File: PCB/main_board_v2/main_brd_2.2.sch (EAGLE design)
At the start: 53 parts, among them J2 SD-card Adapter, J3 E-paper Module, J4 Zigbee Module, J5 BATT, J6 CHARGER, J7 POGO_PINS, J8 ST-LINK, J9 additional I2C bus, U1 STM32F103C8T6-MODULE, U2 LF411CP, U3 TS5A4595DCKR

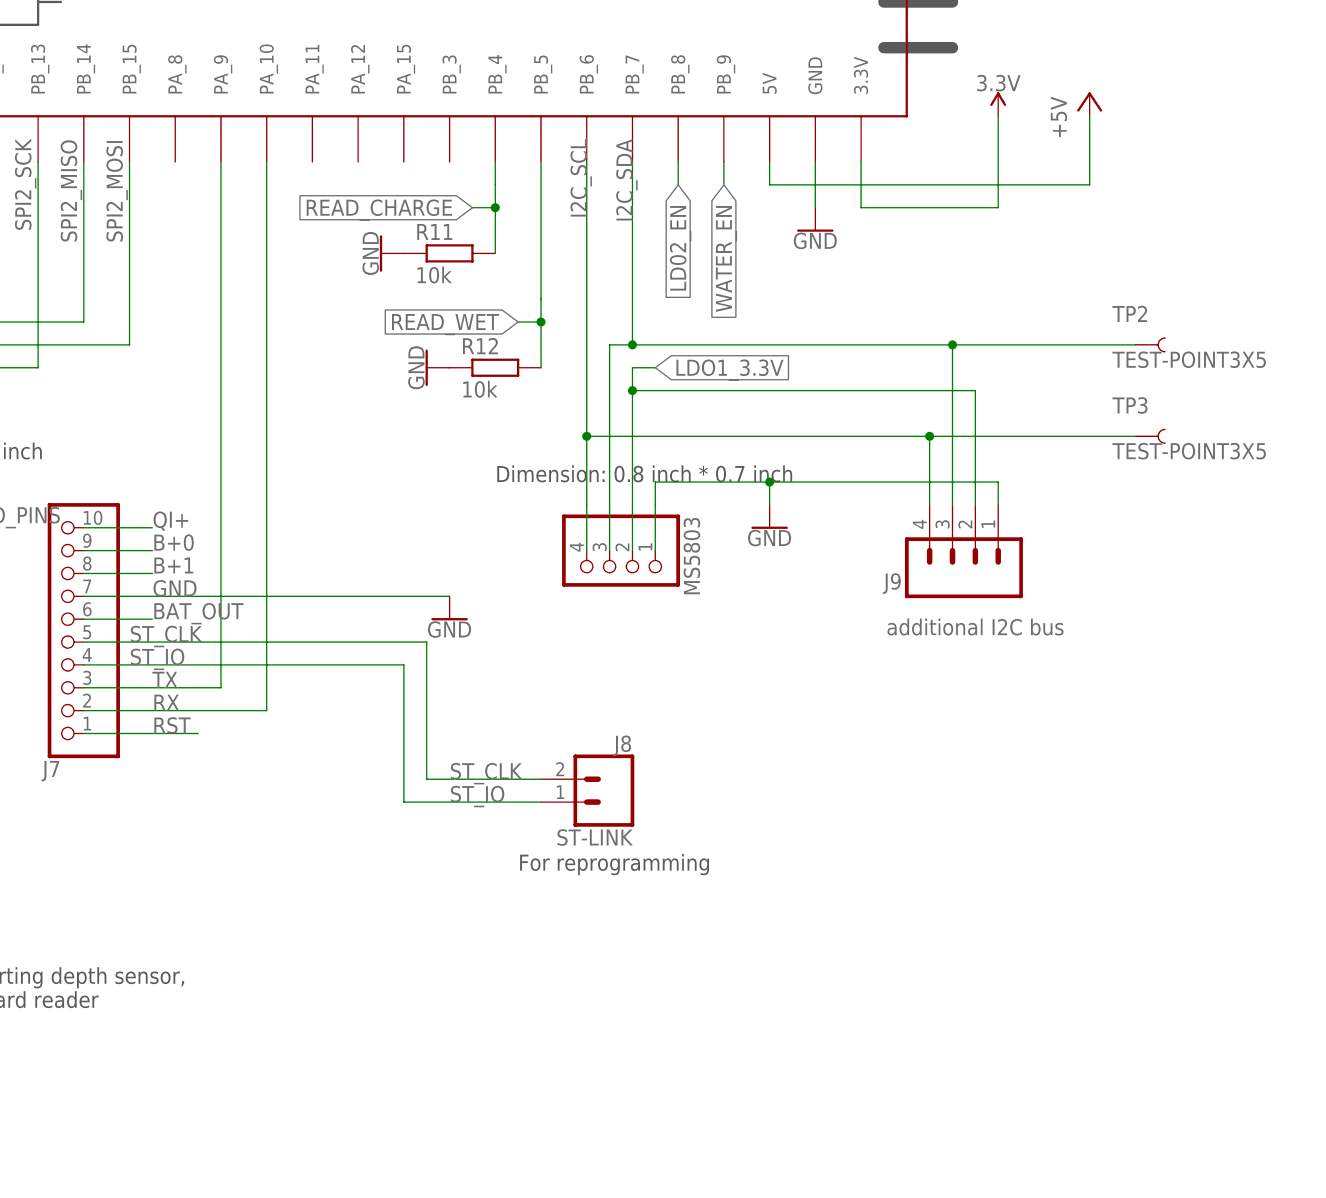
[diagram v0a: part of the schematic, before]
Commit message: Created board 2.2
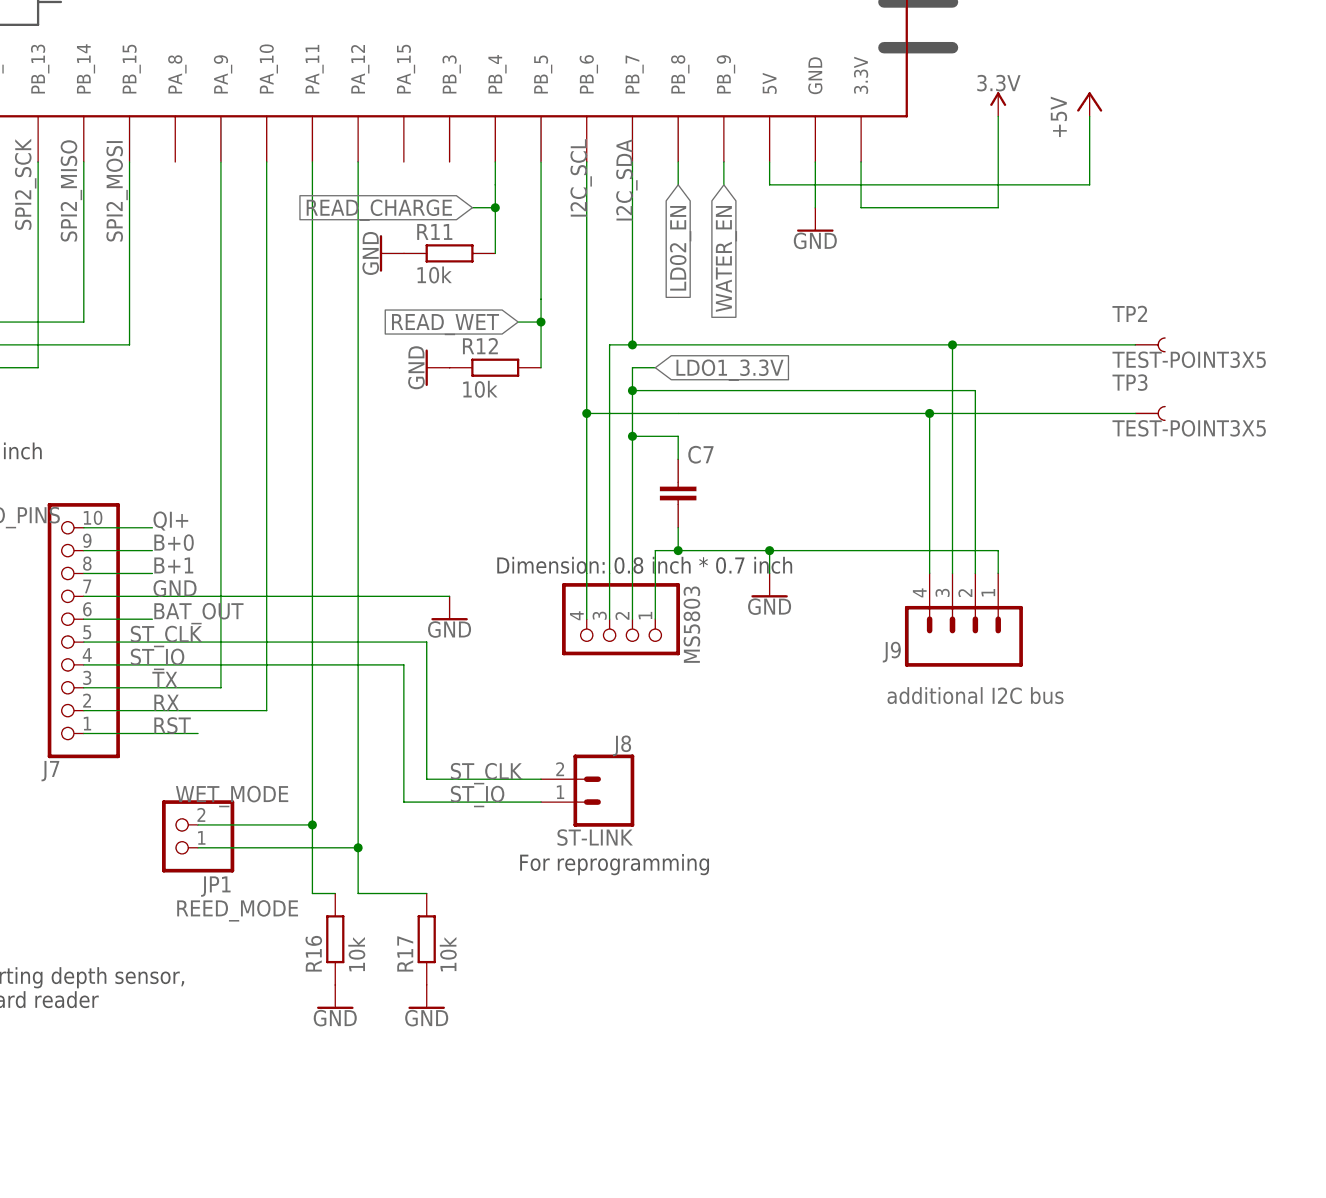
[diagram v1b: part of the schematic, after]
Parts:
- added C7: 100u, rcl:C-EU025-050X050
- added JP1: (no value), pinhead:PINHD-1X2
- added R16, R17: 10k, eagle-ltspice:RR0603
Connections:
- new net REED_MODE: JP1.1, R17.2, U1.PA_12
- new net WET_MODE: JP1.2, R16.2, U1.PA_11
- net GND: now also C7.2, R16.1, R17.1
- net LDO1_3.3V: now also C7.1
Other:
- moved on the sheet: J9, MS5803, TP3
